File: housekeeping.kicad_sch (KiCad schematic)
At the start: 5 parts, among them U2 TPS7B8133QDGNRQ1

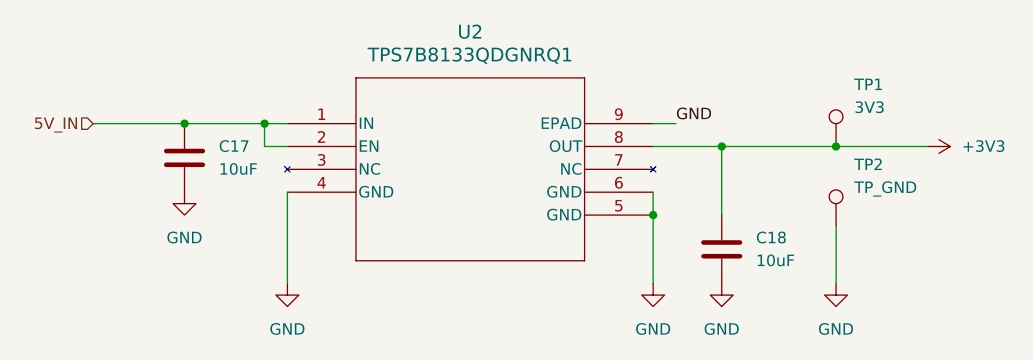
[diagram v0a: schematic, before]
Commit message: Layed on board. Still need to route
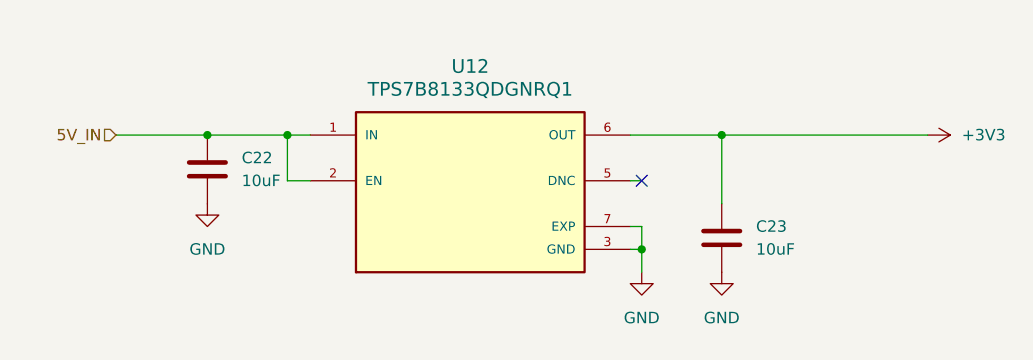
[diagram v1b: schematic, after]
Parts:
- removed C17, C18: 10uF, Capacitor_SMD:C_0805_2012Metric, symbol Device:C
- removed TP1: 3V3, _NavLights:HARWIN_S1751-46R, symbol Connector:TestPoint
- removed TP2: TP_GND, _NavLights:HARWIN_S1751-46R, symbol Connector:TestPoint
- removed U2: TPS7B8133QDGNRQ1, _NavLights:VSSOP8_DGN_TEX, symbol _TPS7B81-Q1:TPS7B8133QDGNRQ1
- added C22, C23: 10uF, Capacitor_SMD:C_0805_2012Metric, symbol Device:C
- added U12: TPS7B8133QDGNRQ1, _BMS:VSSOP8_DGN_TEX, symbol _TPS7B:TPS7B8133DRVR
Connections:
- net +3V3: now also C23.1, U12.6 (OUT)
- net 5V_IN: now also C22.1, U12.1 (IN), U12.2 (EN)
- net GND: now also C22.2, C23.2, U12.3 (GND), U12.4 (GND), U12.7 (EXP)
- no-connect marks 0 -> 1
